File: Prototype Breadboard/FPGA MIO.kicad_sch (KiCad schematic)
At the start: 27 parts, among them U3 XC7Z010-1CLG225I, U5 W25Q128JVS, U6 0473092651, X1 SIT8008BI-73-XXS-33.333333

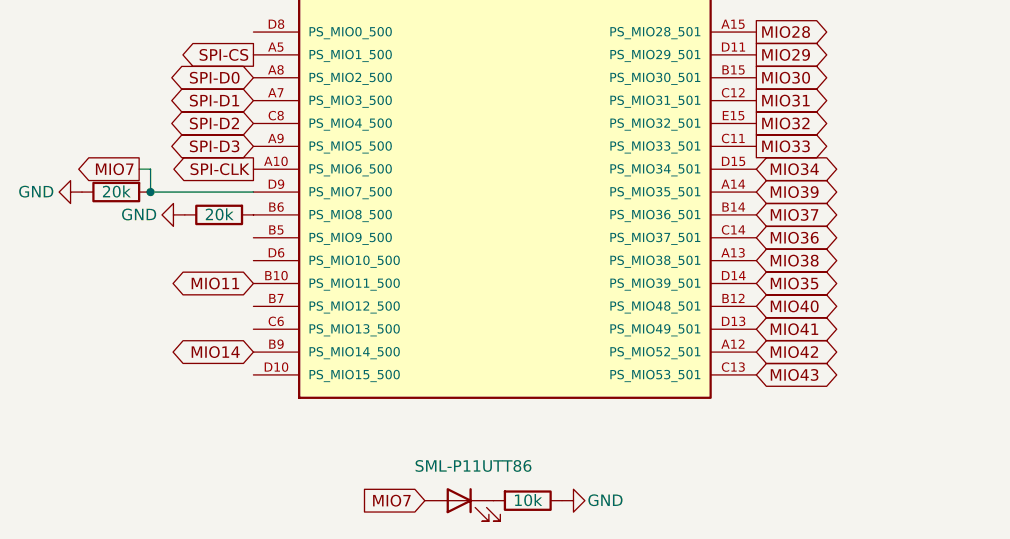
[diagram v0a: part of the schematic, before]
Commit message: 1/4 update
update the breadboard version
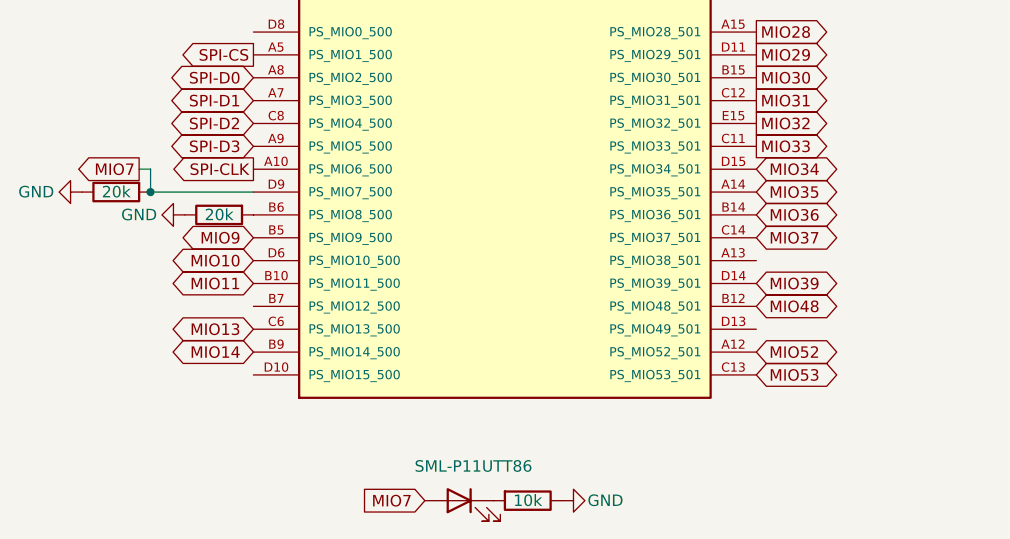
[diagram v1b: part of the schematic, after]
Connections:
- net MIO35: now also U3.A14 (PS_MIO35_501); no longer U3.D14 (PS_MIO39_501)
- net MIO36: now also U3.B14 (PS_MIO36_501); no longer U3.C14 (PS_MIO37_501)
- net MIO37: now also U3.C14 (PS_MIO37_501); no longer U3.B14 (PS_MIO36_501)
- net MIO39: now also U3.D14 (PS_MIO39_501); no longer U3.A14 (PS_MIO35_501)
- net MIO9: now reaches U3.B5 (PS_MIO9_500)
- net MIO13: now reaches U3.C6 (PS_MIO13_500)
- net MIO10: now reaches U3.D6 (PS_MIO10_500)
- net MIO38: no longer names the net of U3.A13 (PS_MIO38_501)
- net MIO40 renamed MIO48
- net MIO41: no longer names the net of U3.D13 (PS_MIO49_501)
- net MIO42 renamed MIO52
- net MIO43 renamed MIO53
